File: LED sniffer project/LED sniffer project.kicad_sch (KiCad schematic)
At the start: 13 parts, among them J1 Conn_01x02_Pin, Q1 2N3904, SW1 Push_Button

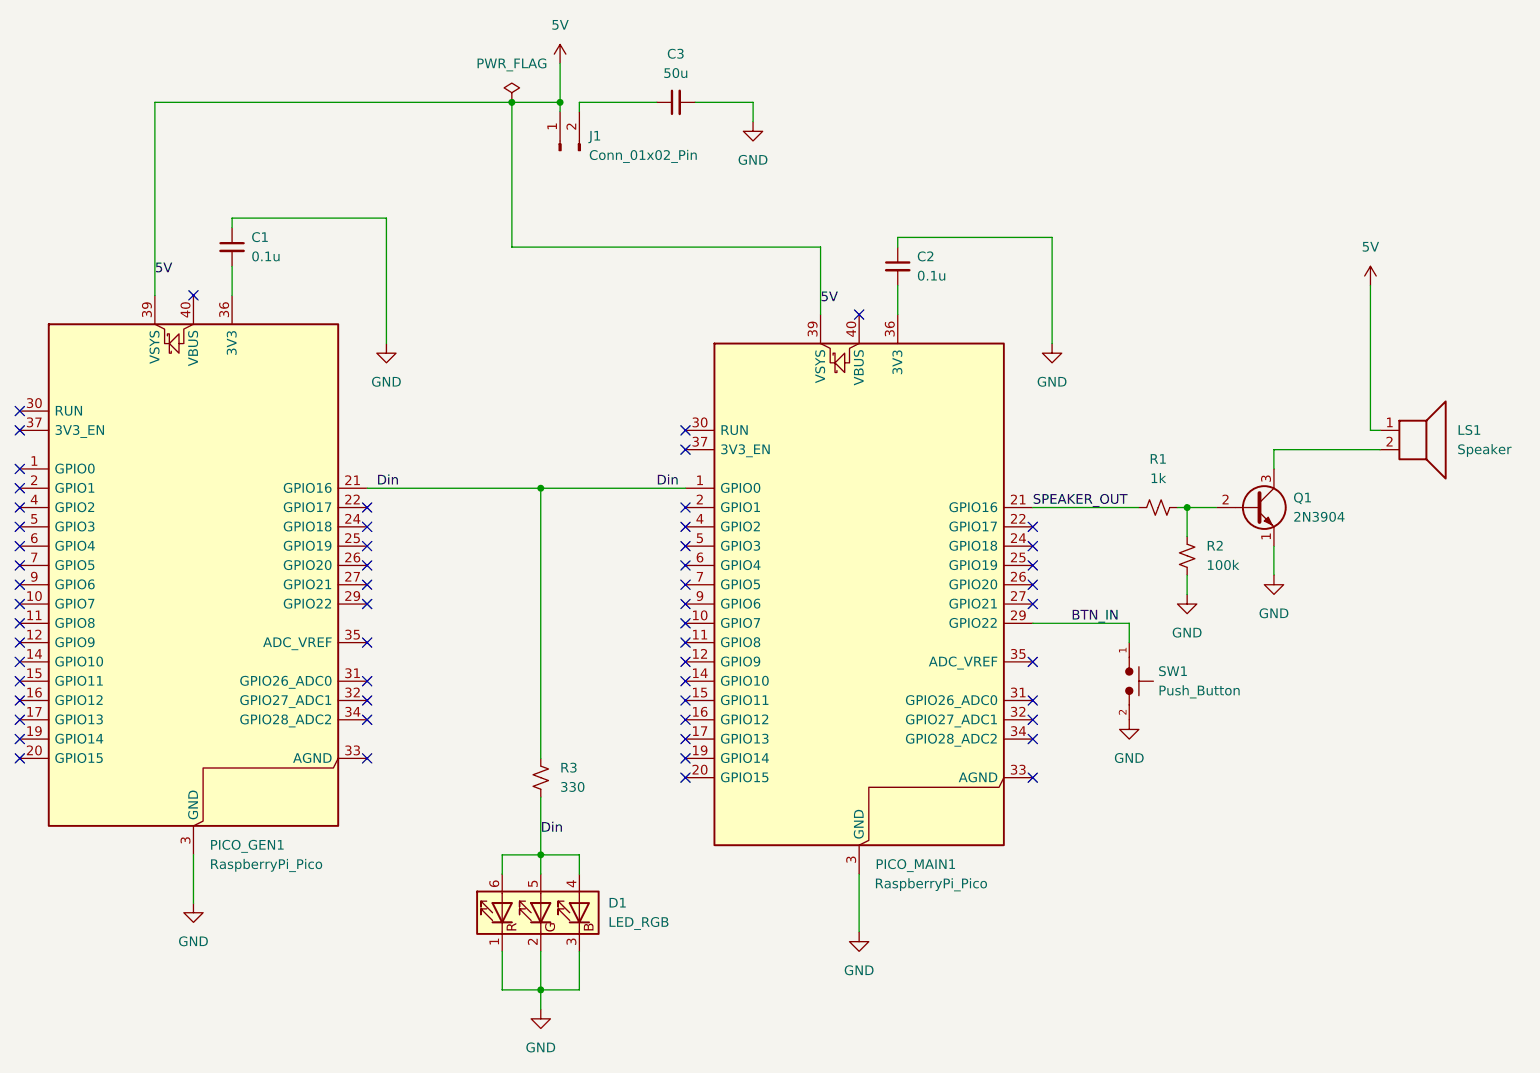
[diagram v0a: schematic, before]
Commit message: rough draft of schematic
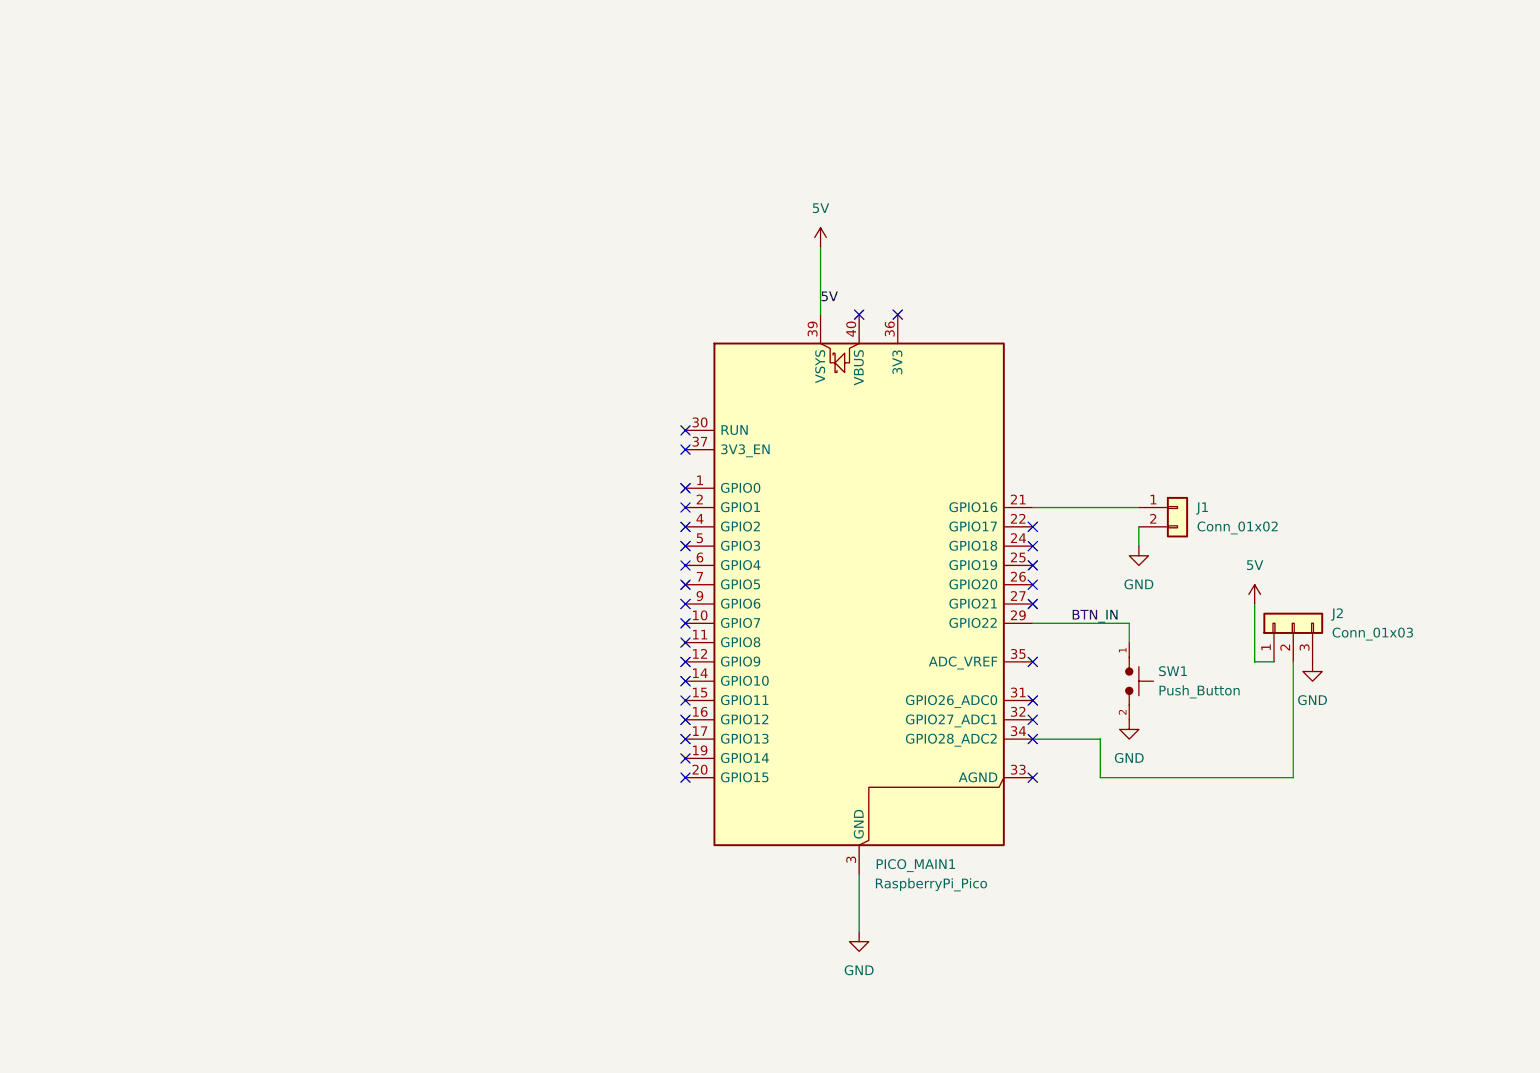
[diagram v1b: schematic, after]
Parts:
- removed C1, C2: 0.1u, Capacitor_SMD:C_1206_3216Metric, symbol Device:C_Small
- removed C3: 50u, Capacitor_SMD:C_1206_3216Metric, symbol Device:C_Small
- removed D1: LED_RGB, LED_SMD:LED_RGB_PLCC-6, symbol Device:LED_RGB
- removed J1: Conn_01x02_Pin, Connector_PinHeader_2.54mm:PinHeader_1x02_P2.54mm_Vertical, symbol Connector:Conn_01x02_Pin
- removed LS1: Speaker, Connector_PinHeader_2.54mm:PinHeader_1x02_P2.54mm_Vertical, symbol Device:Speaker
- removed PICO_GEN1: RaspberryPi_Pico, Module:RaspberryPi_Pico_Common_Unspecified, symbol MCU_Module:RaspberryPi_Pico
- removed Q1: 2N3904, Package_TO_SOT_THT:TO-92_Inline, symbol Transistor_BJT:2N3904
- removed R1: 1k, Resistor_SMD:R_1206_3216Metric, symbol Device:R_Small_US
- removed R2: 100k, Resistor_SMD:R_1206_3216Metric, symbol Device:R_Small_US
- removed R3: 330, Resistor_SMD:R_1206_3216Metric, symbol Device:R_Small_US
- added J1: Conn_01x02, Connector_PinHeader_1.00mm:PinHeader_1x02_P1.00mm_Vertical, symbol PCM_4ms_Connector:Conn_01x02
- added J2: Conn_01x03, Connector_PinHeader_1.00mm:PinHeader_1x03_P1.00mm_Vertical, symbol PCM_4ms_Connector:Conn_01x03
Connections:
- net 5V: now also J2.1 (Pin_1)
- net GND: now also J1.2 (Pin_2), J2.3 (Pin_3)
- net at PICO_MAIN1.34 (GPIO28_ADC2): now also J2.2 (Pin_2)
- net Din: no longer names the net of PICO_MAIN1.1 (GPIO0)
- net SPEAKER_OUT: no longer names the net of PICO_MAIN1.21 (GPIO16)
- net SPEAKER_OUT: now also J1.1 (Pin_1)
- no-connect marks 58 -> 30

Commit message: Updated with a slightly less rough draft
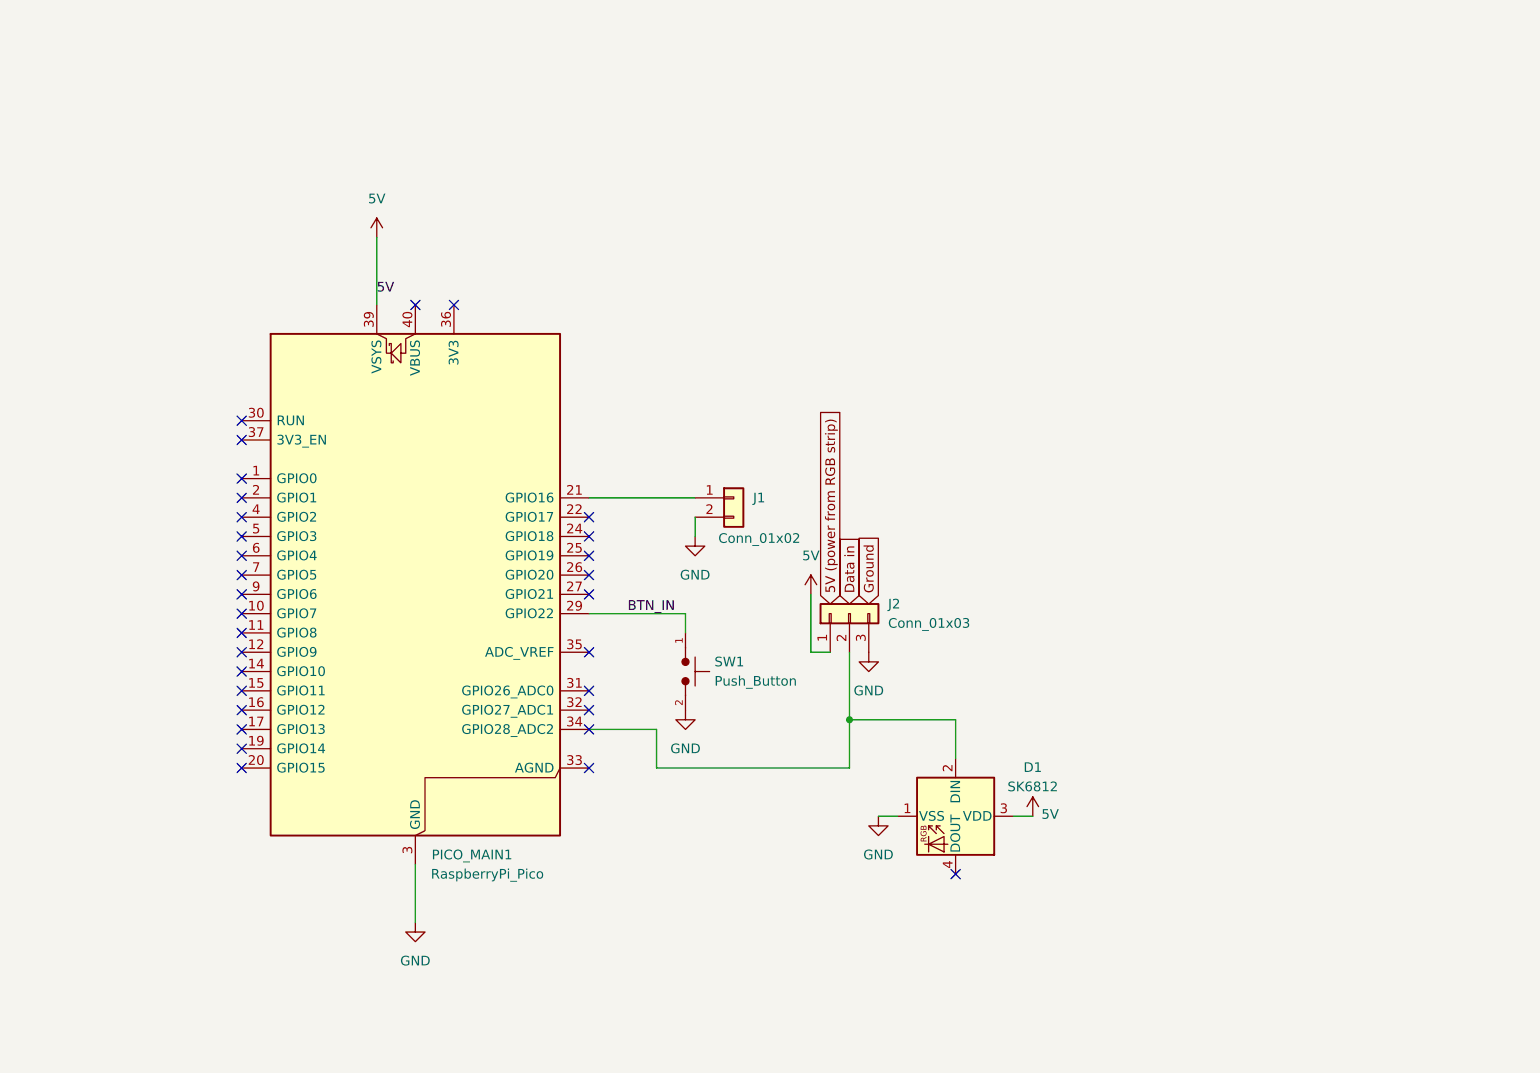
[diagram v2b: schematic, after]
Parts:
- added D1: SK6812, LED_SMD:LED_SK6812_PLCC4_5.0x5.0mm_P3.2mm, symbol LED:SK6812
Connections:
- net 5V: now also D1.3 (VDD)
- net GND: now also D1.1 (VSS)
- net at J2.2 (Pin_2), PICO_MAIN1.34 (GPIO28_ADC2): now also D1.2 (DIN)
- no-connect marks 30 -> 31
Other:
- company: (none) -> Team 09
- moved on the sheet: J1, J2, PICO_MAIN1, SW1

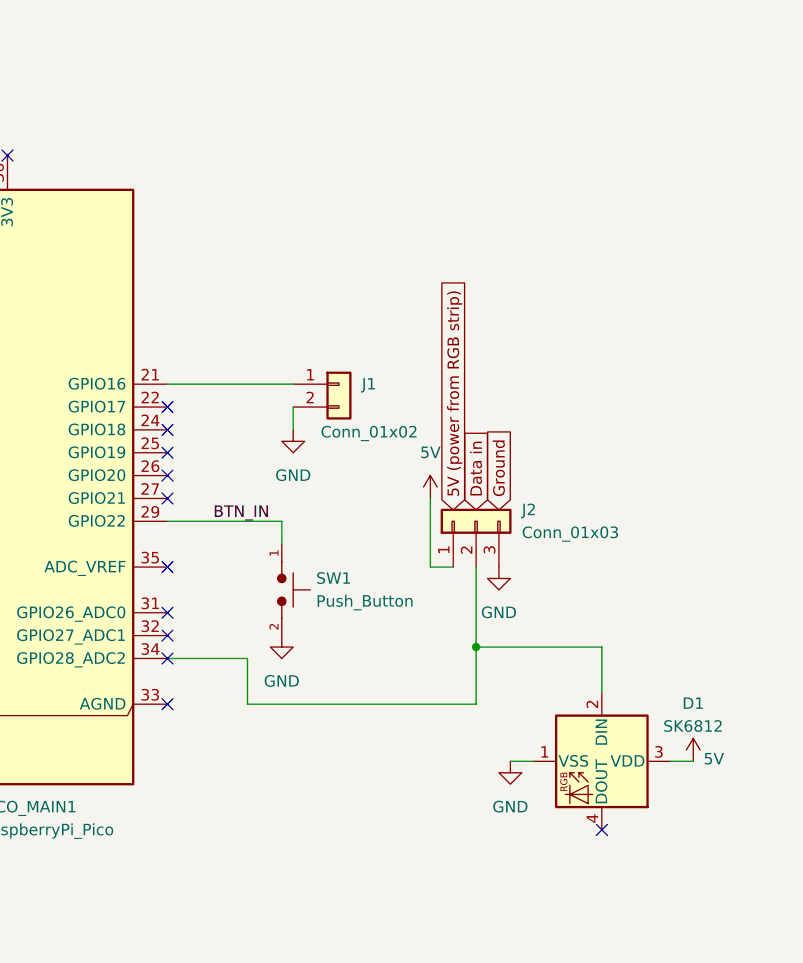
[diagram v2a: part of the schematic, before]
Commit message: Updated CAD
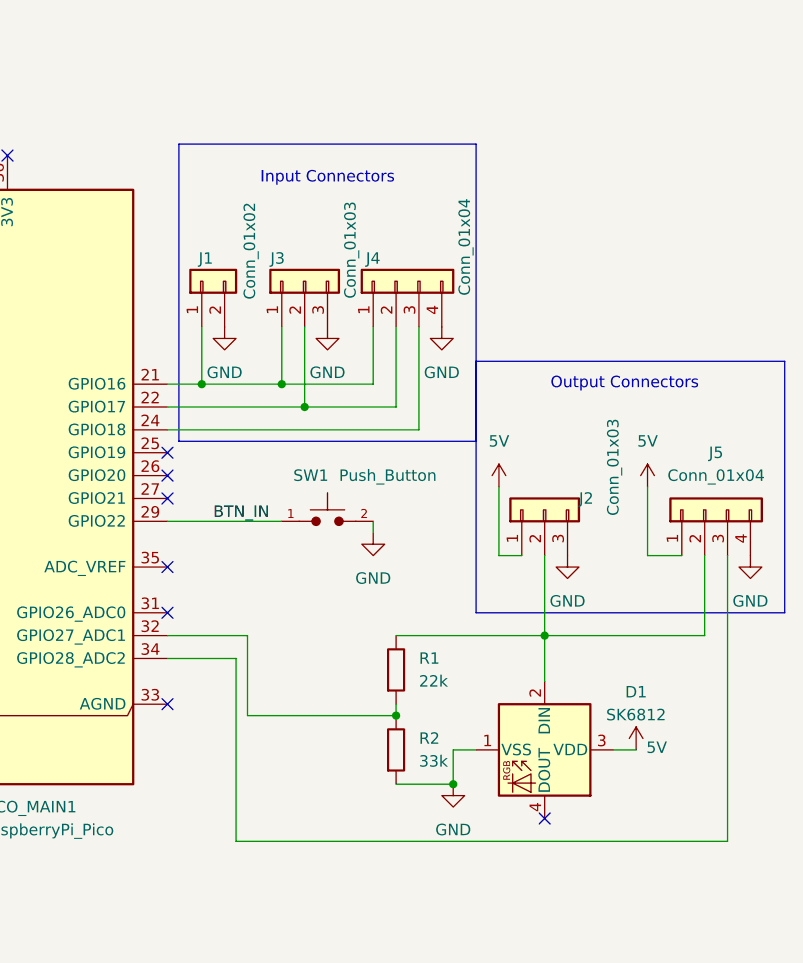
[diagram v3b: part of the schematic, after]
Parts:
- added J3: Conn_01x03, Connector_PinHeader_2.54mm:PinHeader_1x03_P2.54mm_Vertical, symbol PCM_4ms_Connector:Conn_01x03
- added J4, J5: Conn_01x04, Connector_PinHeader_2.54mm:PinHeader_1x04_P2.54mm_Vertical, symbol PCM_4ms_Connector:Conn_01x04
- added R1: 22k, Resistor_THT:R_Axial_DIN0207_L6.3mm_D2.5mm_P10.16mm_Horizontal, symbol PCM_SL_Resistors:22k
- added R2: 33k, Resistor_THT:R_Axial_DIN0207_L6.3mm_D2.5mm_P10.16mm_Horizontal, symbol PCM_SL_Resistors:33k
- J1: footprint Connector_PinHeader_1.00mm:PinHeader_1x02_P1.00mm_Vertical -> Connector_PinHeader_2.54mm:PinHeader_1x02_P2.54mm_Vertical
- J2: footprint Connector_PinHeader_1.00mm:PinHeader_1x03_P1.00mm_Vertical -> Connector_PinHeader_2.54mm:PinHeader_1x03_P2.54mm_Vertical
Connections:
- net 5V: now also J5.1 (Pin_1)
- net GND: now also J3.3 (Pin_3), J4.4 (Pin_4), J5.4 (Pin_4), R2.1
- net at J1.1 (Pin_1), PICO_MAIN1.21 (GPIO16): now also J3.1 (Pin_1), J4.1 (Pin_1)
- net at PICO_MAIN1.22 (GPIO17): now also J3.2 (Pin_2), J4.2 (Pin_2)
- net at PICO_MAIN1.24 (GPIO18): now also J4.3 (Pin_3)
- net at PICO_MAIN1.32 (GPIO27_ADC1): now also R1.1, R2.2
- net at D1.2 (DIN), J2.2 (Pin_2): now also J5.2 (Pin_2), R1.2; no longer PICO_MAIN1.34 (GPIO28_ADC2)
- new net: J5.3 (Pin_3), PICO_MAIN1.34 (GPIO28_ADC2)
- no-connect marks 31 -> 27
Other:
- note added: "Input Connectors"
- note added: "Output Connectors"
- moved on the sheet: D1, J1, J2, SW1
